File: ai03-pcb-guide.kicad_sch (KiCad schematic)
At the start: 16 parts, among them J1 AVR-ISP-6, SW1 SW_Push, U1 ATmega32U4-A, Y1 16MHz

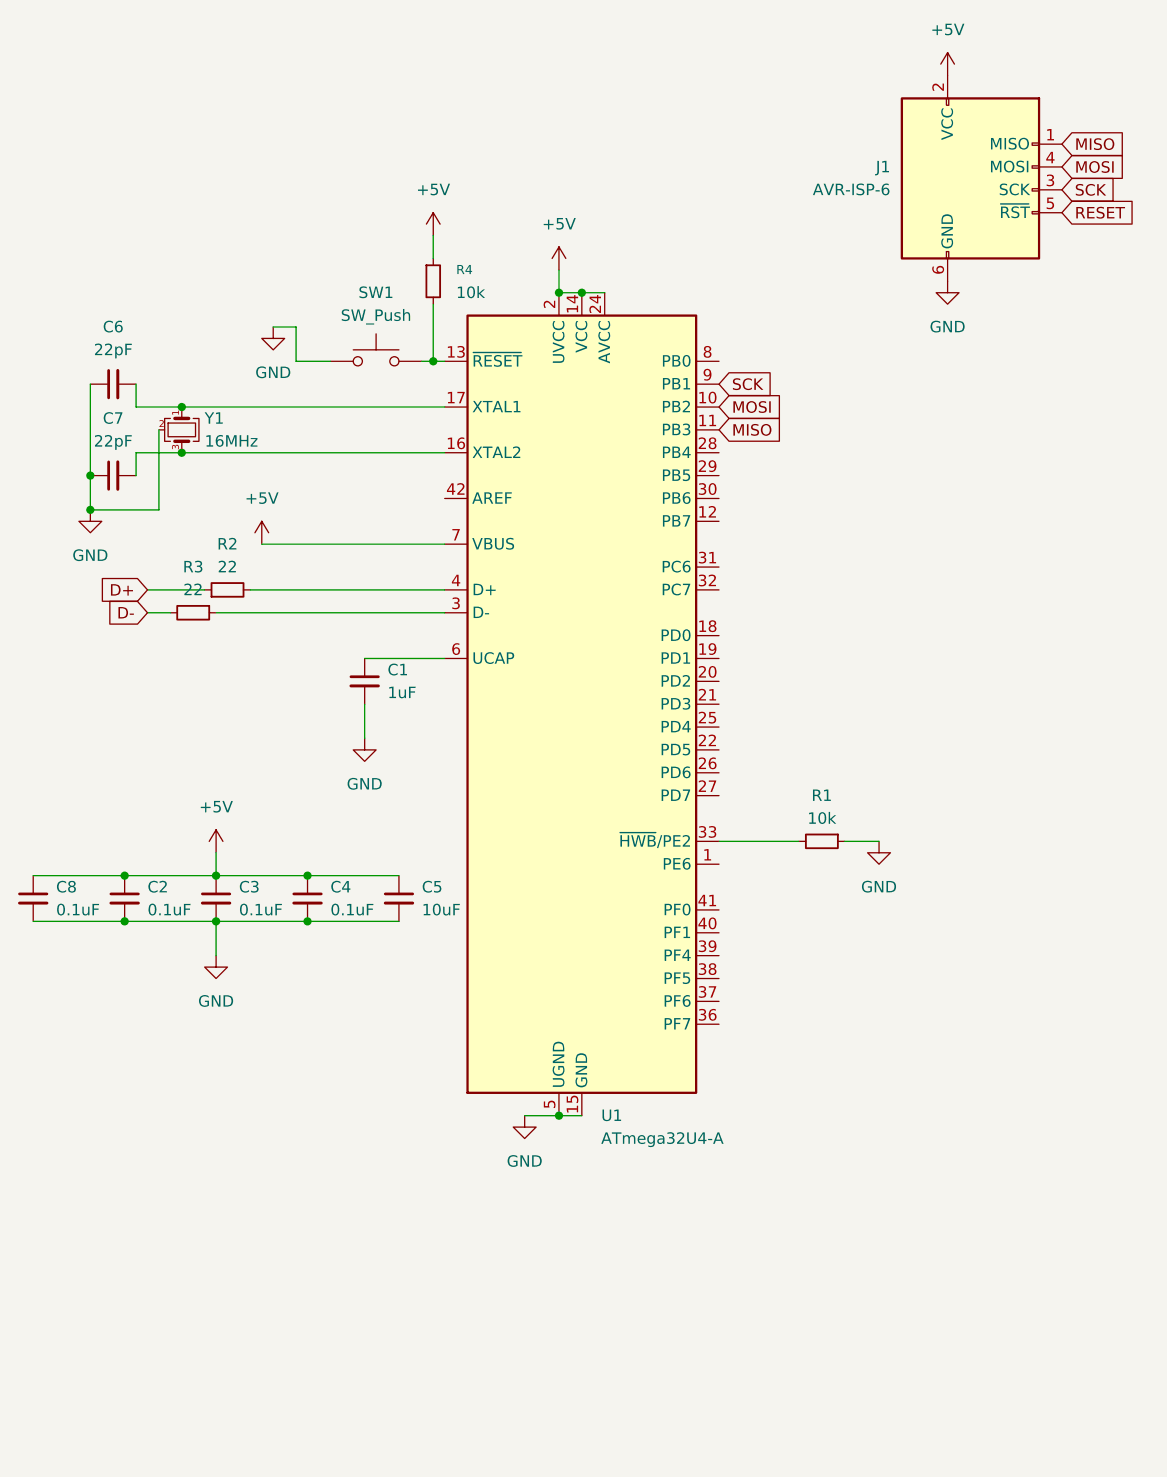
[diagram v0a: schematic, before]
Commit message: more MCU schema
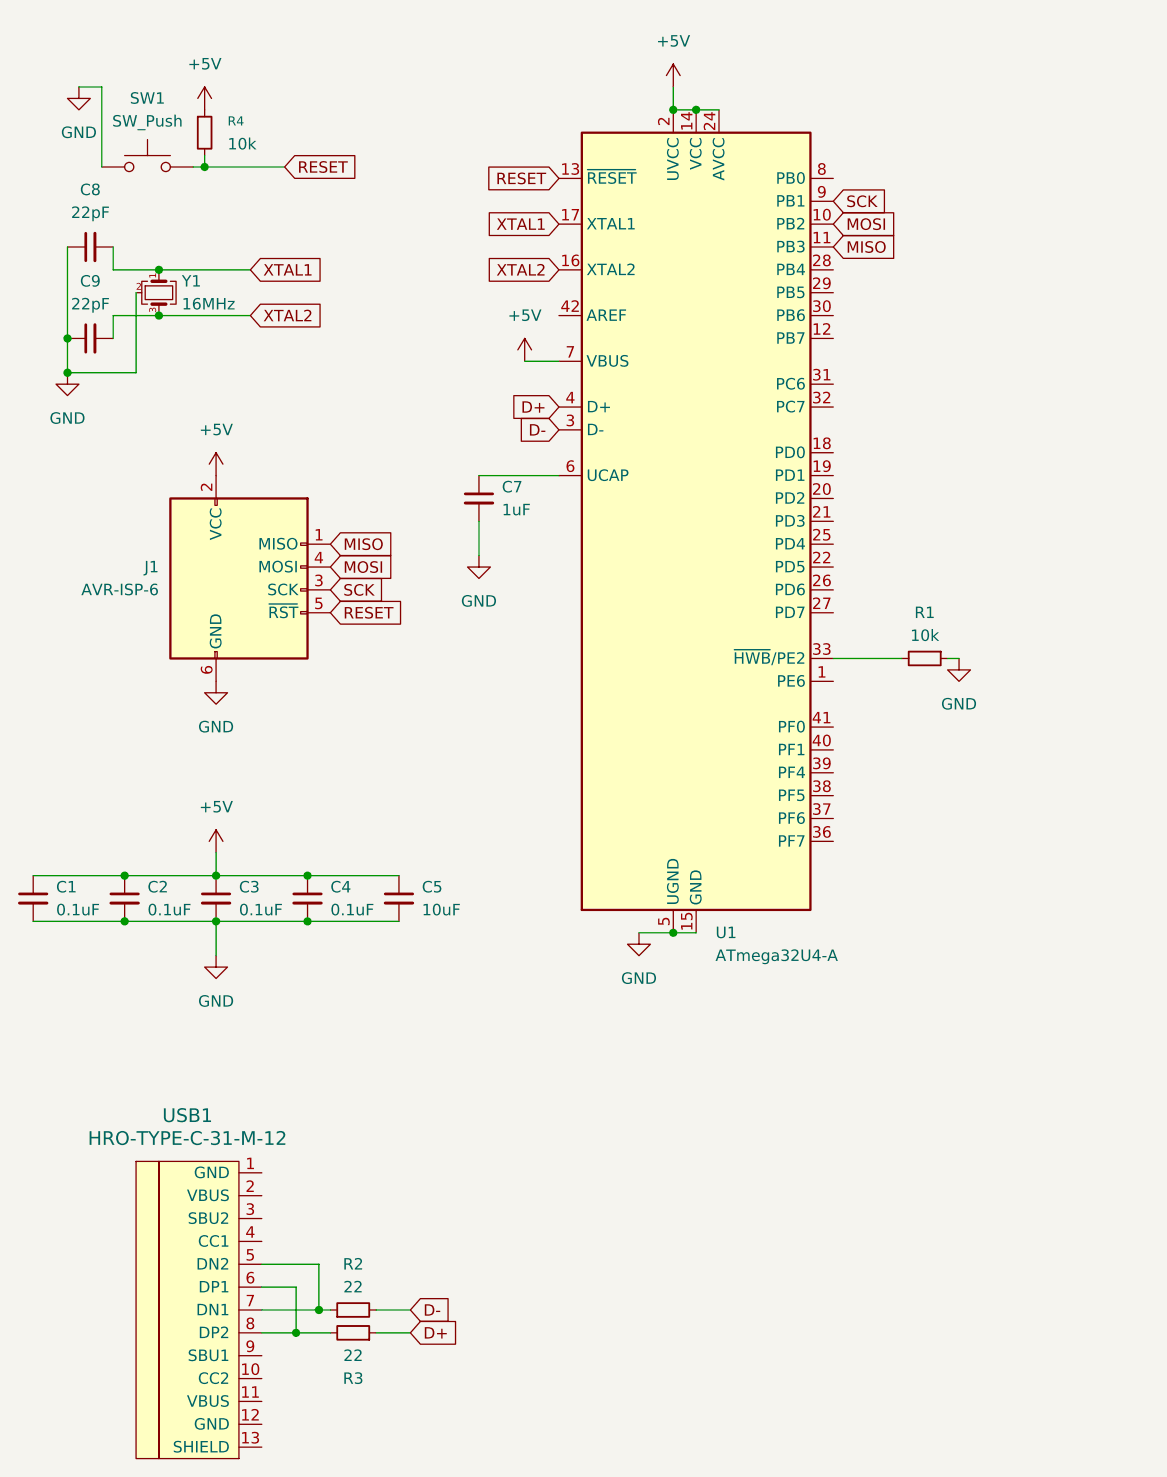
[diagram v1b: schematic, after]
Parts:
- added USB1: HRO-TYPE-C-31-M-12, symbol Type-C:HRO-TYPE-C-31-M-12
- renumbered C8 to C1, C1 to C7, C6 to C8, C7 to C9
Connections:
- net D+: now also R3.1, U1.4 (D+); no longer R2.1
- net D-: now also R2.2, U1.3 (D-); no longer R3.2
- net RESET: now also R4.2, SW1.2, U1.13 (~{RESET})
- net XTAL1: now reaches C8.2, U1.17 (XTAL1), Y1.1
- net XTAL2: now reaches C9.2, U1.16 (XTAL2), Y1.3
- new net: R3.2, USB1.6 (DP1), USB1.8 (DP2)
- new net: R2.1, USB1.5 (DN2), USB1.7 (DN1)
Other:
- moved on the sheet: C7, C8, C9, J1, R1, R2, R3, R4, SW1, U1, Y1
